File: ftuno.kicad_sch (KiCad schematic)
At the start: 66 parts, among them CN1 AFC10-S04QCA-00, J1 Conn_01x08_Pin, J10 Conn_02x04_Odd_Even, J11 Conn_01x04_Socket, J2 Conn_01x08_Socket, J3 Conn_01x06_Pin, J4 Conn_01x06_Socket, J5 Conn_01x10_Pin, J6 Conn_01x10_Socket, J7 Conn_01x08_Pin, J8 Conn_01x08_Socket, J9 Conn_02x03_Odd_Even, Q1 AO3401, Q2 BSS138PS_C5224289, Q3 BSS138PS_C5224289, SW1 SK12D07VG4, SW2 TS-1187A-B-A-B, U1 ATmega328P-A, U2 CH340C, U3 SRV05-4, U4 TPS54302, U5 ME6217C33M5G, X1 CSTCE16M0V53-R0

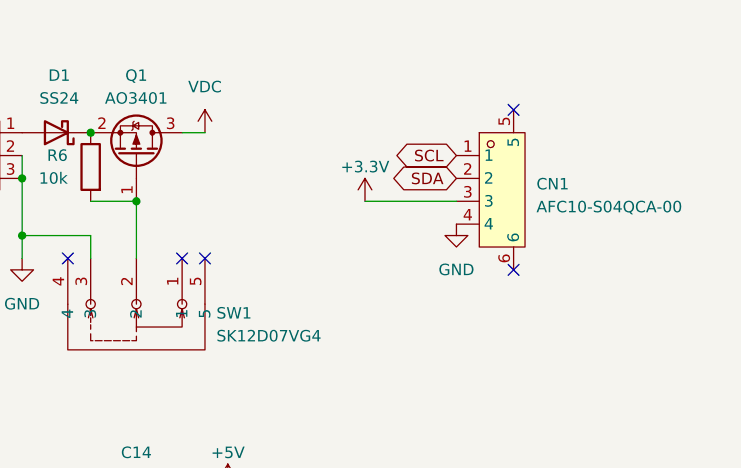
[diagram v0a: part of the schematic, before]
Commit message: fix qwiic
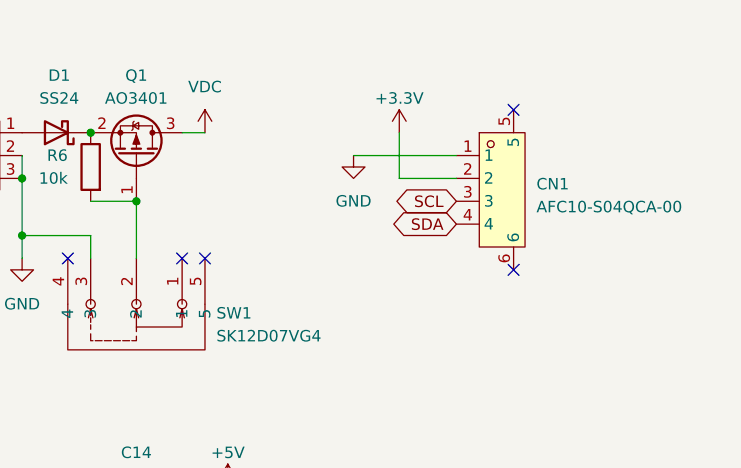
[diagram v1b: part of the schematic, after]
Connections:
- net +3.3V: now also CN1.2; no longer CN1.3
- net GND: now also CN1.1; no longer CN1.4
- net SCL: now also CN1.3; no longer CN1.1
- net SDA: now also CN1.4; no longer CN1.2
